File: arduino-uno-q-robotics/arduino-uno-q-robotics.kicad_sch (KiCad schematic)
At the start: 19 parts, among them J1 Conn_02x30_Odd_Even, J2 Conn_02x30_Odd_Even, J3 Connector_FFC-FPC, J4 Connector_FFC-FPC, J5 Conn_02x13_Odd_Even, J6 Conn_02x04_Odd_Even, U1 LSM6DSO32, U2 TCA9803, U4 TCA9803

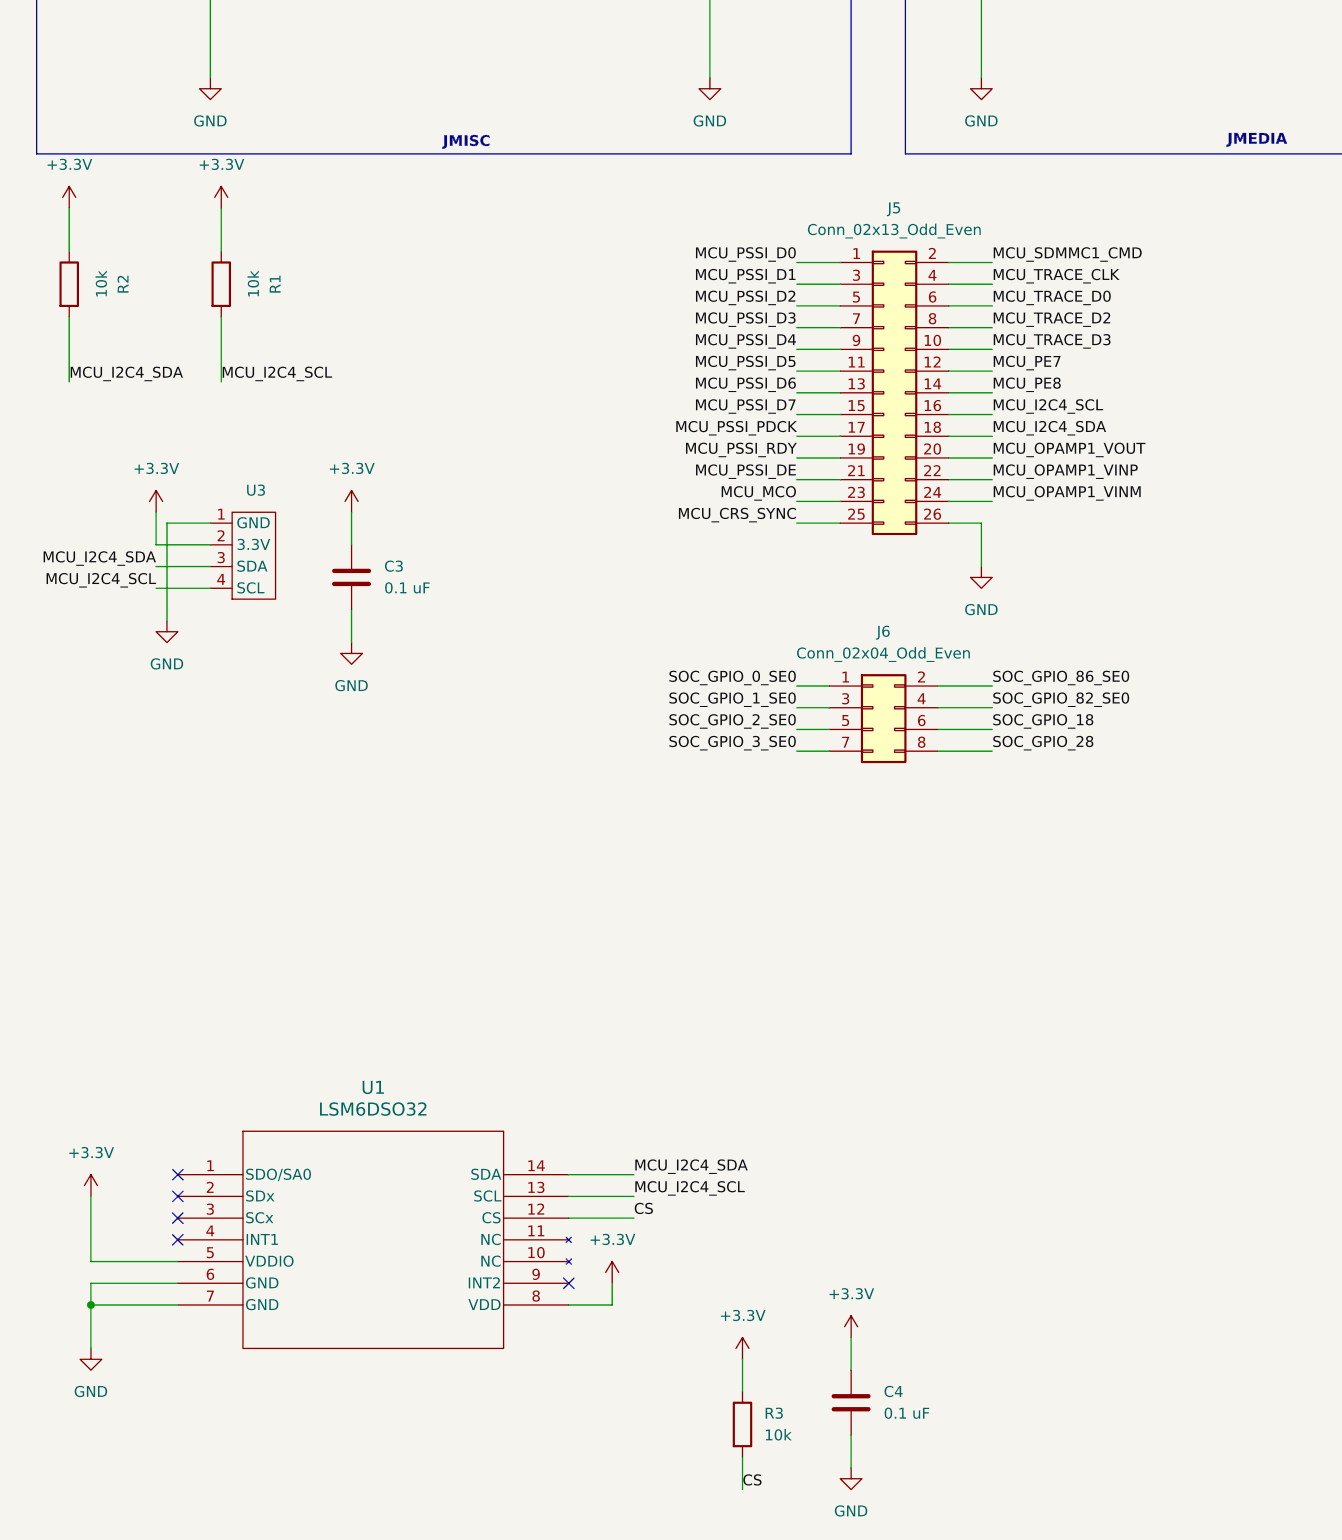
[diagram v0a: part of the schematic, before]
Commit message: Organize schematic sheet
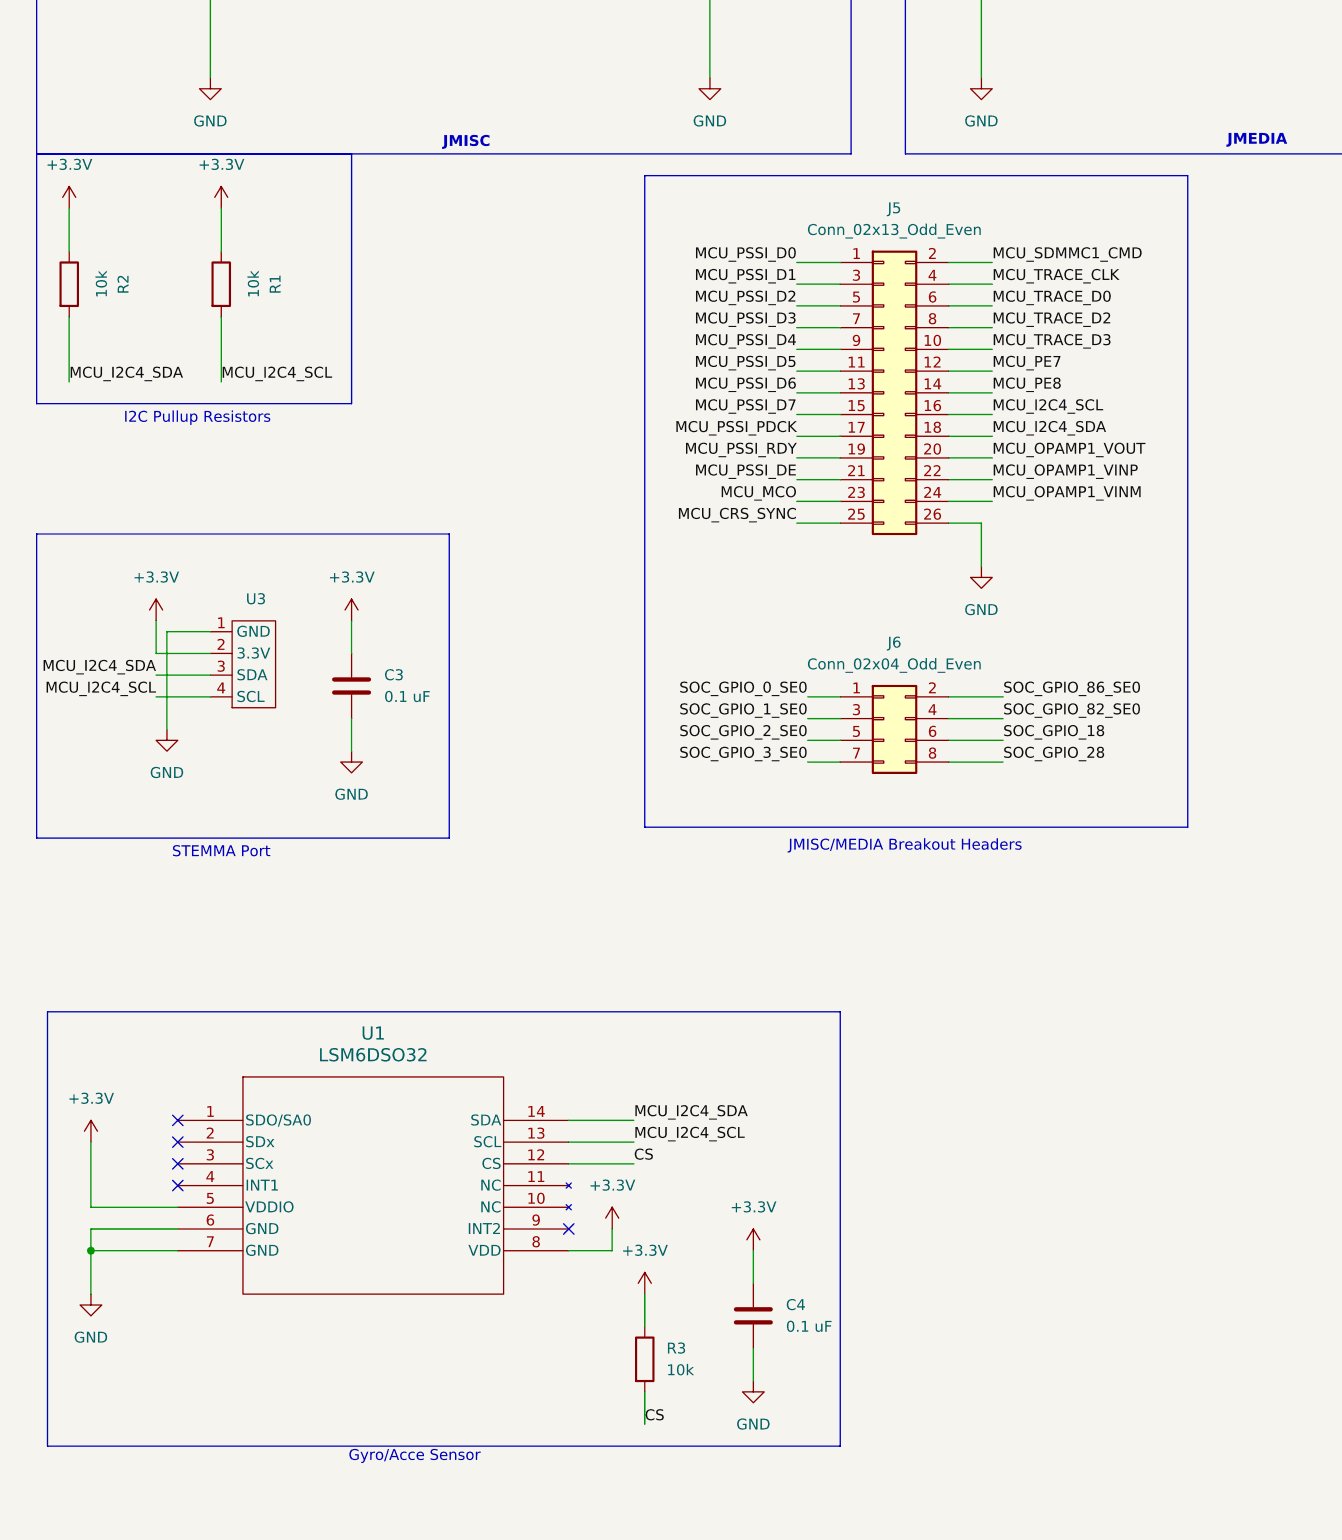
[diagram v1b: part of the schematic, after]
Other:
- note added: "Gyro/Acce Sensor"
- note added: "I2C Pullup Resistors"
- note added: "JMISC/MEDIA Breakout Headers"
- note added: "STEMMA Port"
- moved on the sheet: C3, C4, J6, R3, U1, U3
